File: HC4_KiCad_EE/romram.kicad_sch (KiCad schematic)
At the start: 5 parts, among them J1 Conn_02x04_Odd_Even, J4 UPDI_and_Debug, U1 ATmega4809-A

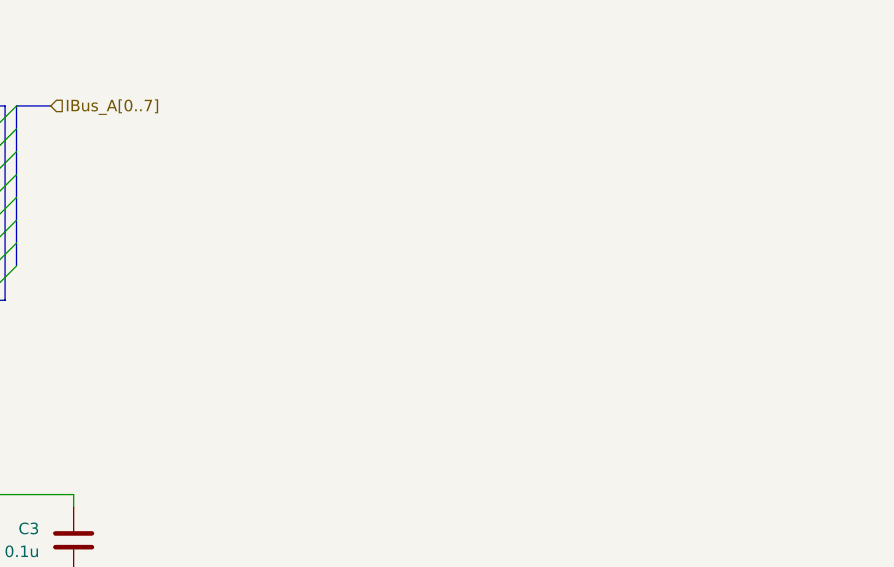
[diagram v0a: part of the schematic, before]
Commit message: 基板に反映
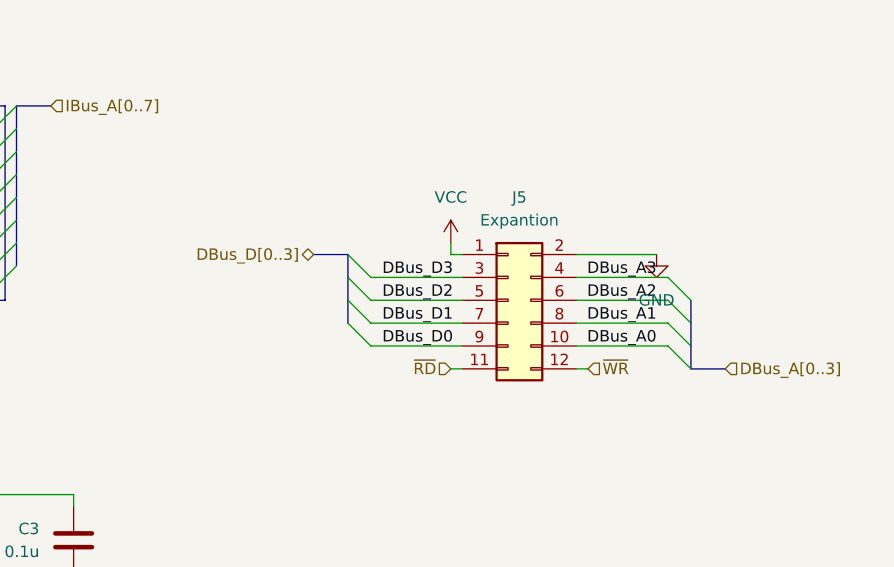
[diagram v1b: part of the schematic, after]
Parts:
- added J5: Expantion, Connector_PinHeader_2.54mm:PinHeader_2x06_P2.54mm_Vertical, symbol Connector_Generic:Conn_02x06_Odd_Even
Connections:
- net DBus_A0: now also J5.10 (Pin_10)
- net DBus_A1: now also J5.8 (Pin_8)
- net DBus_A2: now also J5.6 (Pin_6)
- net DBus_A3: now also J5.4 (Pin_4)
- net DBus_D0: now also J5.9 (Pin_9)
- net DBus_D1: now also J5.7 (Pin_7)
- net DBus_D2: now also J5.5 (Pin_5)
- net DBus_D3: now also J5.3 (Pin_3)
- net GND: now also J5.2 (Pin_2)
- net VCC: now also J5.1 (Pin_1)
- net ~{RD}: now also J5.11 (Pin_11)
- net ~{WR}: now also J5.12 (Pin_12)
